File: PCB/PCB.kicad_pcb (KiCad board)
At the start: 2 copper layers, 85 x 55 mm, 32 parts, among them IC2 AP33771CFBZ-13-FA01, IC3 LT8609EMSE#PBF, IC4 AP63203WU-7, J3 UJ20-C-V-SMT-TR-68, Q1 PSMN2R6-30YLC,115, Q2 PSMN2R6-30YLC,115

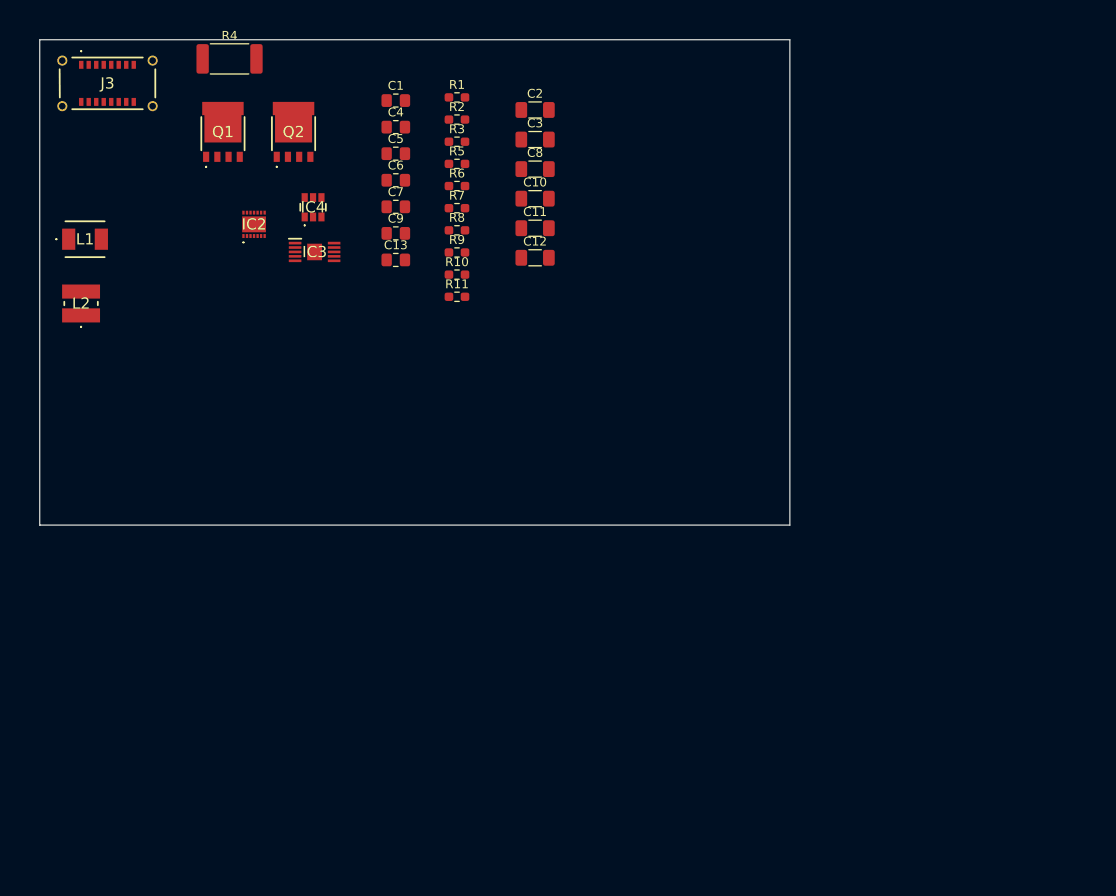
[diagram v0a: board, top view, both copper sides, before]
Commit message: backup power rail pcb
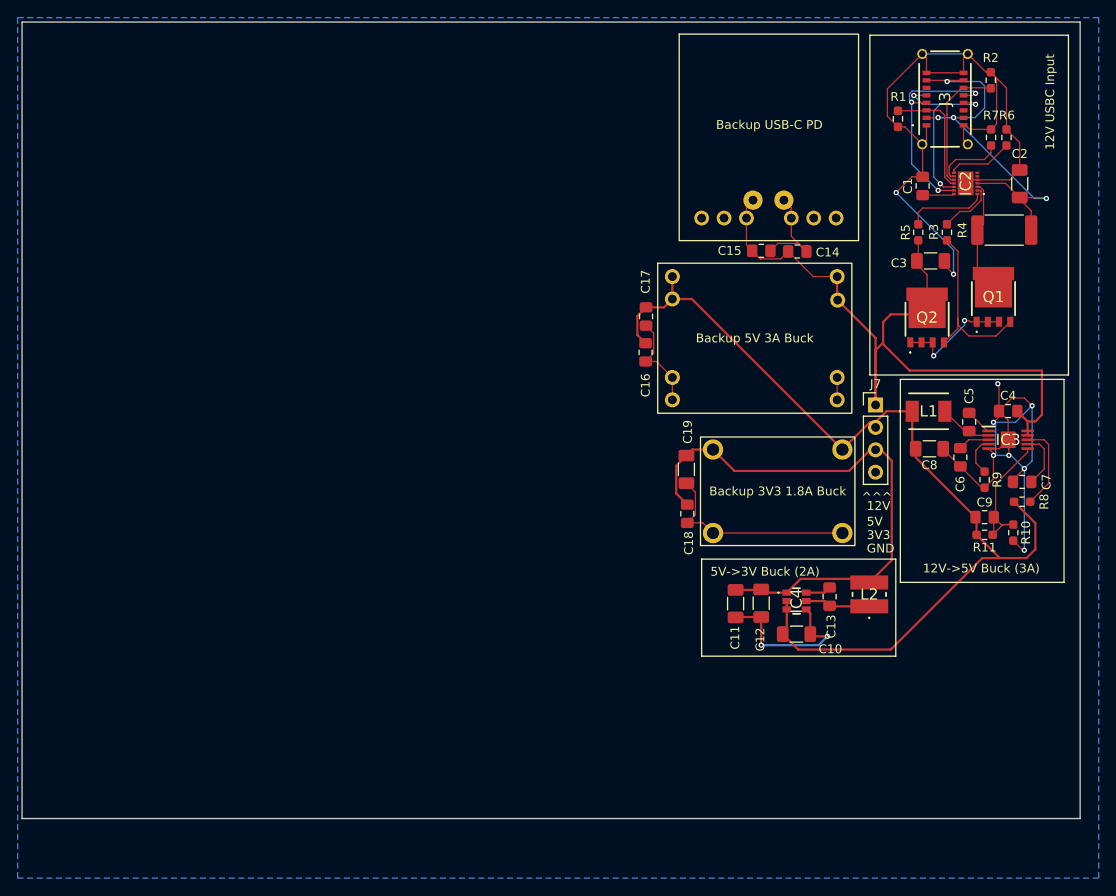
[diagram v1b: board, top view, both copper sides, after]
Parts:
- added C14: 0.1uF, Capacitor_SMD:C_0805_2012Metric_Pad1.18x1.45mm_HandSolder, F.Cu at (100.8, 39.0)
- added C15: 47uF, Capacitor_SMD:C_0805_2012Metric_Pad1.18x1.45mm_HandSolder, F.Cu at (96.8, 38.9)
- added C16: 0.1uF, Capacitor_SMD:C_0805_2012Metric_Pad1.18x1.45mm_HandSolder, F.Cu at (83.7, 50.4)
- added C17: 47uF, Capacitor_SMD:C_0805_2012Metric_Pad1.18x1.45mm_HandSolder, F.Cu at (83.7, 46.4)
- added C18: 0.1uF, Capacitor_SMD:C_0805_2012Metric_Pad1.18x1.45mm_HandSolder, F.Cu at (88.4, 68.7)
- added C19: 22uF, Capacitor_SMD:C_1206_3216Metric_Pad1.33x1.80mm_HandSolder, F.Cu at (88.3, 63.7)
- added J6: USBC_Power_Breakout, SpinnyKitty:USBC_POWER_BREAKOUT, F.Cu at (97.6, 33.2)
- added J7: ~, Connector_PinHeader_2.54mm:PinHeader_1x04_P2.54mm_Vertical, F.Cu at (109.7, 56.4)
- added U3: ~, SpinnyKitty:5V 3A Buck, F.Cu at (96.0, 48.8)
- added U4: ~, SpinnyKitty:3V3 1.8A Buck, F.Cu at (98.6, 66.2)
- C13: value 100nF -> 0.1uF
- moved L1 97.6 mm to (115.7, 57.1)
- moved L2 95.2 mm to (109.0, 77.9)
- moved J3 94.9 mm to (117.6, 21.7), turned to 90 degrees
- moved R4 89.9 mm to (124.3, 36.6), turned to 180 degrees
- moved Q1 89.3 mm to (123.1, 44.3)
- moved IC3 81.4 mm to (124.7, 60.3)
- moved IC2 80.8 mm to (119.9, 31.3), turned to 90 degrees
- moved C7 77.5 mm to (126.3, 65.1)
- moved C4 76.5 mm to (124.7, 57.1), turned to 180 degrees
- moved Q2 74.8 mm to (115.6, 46.6)
- moved C9 74.1 mm to (122.1, 69.1)
- moved C5 71.7 mm to (120.3, 58.3), turned to -90 degrees
- moved C6 71.3 mm to (119.3, 62.3), turned to 90 degrees
- moved R8 71.0 mm to (126.3, 67.4)
- moved IC4 70.7 mm to (100.8, 78.6), turned to -90 degrees
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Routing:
- net GND: track 0.00 -> 217.6 mm, vias 0 -> 11
- net +5V: track 0.00 -> 112.1 mm
- net +12V: track 0.00 -> 84.3 mm
- net +3V3: track 0.00 -> 64.1 mm
- net /VBUS: track 0.00 -> 48.8 mm, vias 0 -> 4
- net /DP: track 0.00 -> 25.0 mm, vias 0 -> 3
- net /DN: track 0.00 -> 21.6 mm, vias 0 -> 3
- net /GATE_DRV: track 0.00 -> 20.6 mm
- net Net-(IC3-FB): track 0.00 -> 16.8 mm
- net /IC_CC2: track 0.00 -> 15.0 mm
- net /IC_CC1: track 0.00 -> 13.9 mm
- net /VBUS_SW_IN: track 0.00 -> 13.6 mm
- net /FET_MID: track 0.00 -> 13.5 mm, vias 0 -> 2
- net /POWER GOOD: track 0.00 -> 9.95 mm
- net Net-(IC2-VOUT): track 0.00 -> 9.28 mm
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- added copper zone on B.Cu, net GND
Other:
- board size 85 x 55 mm -> 119.9 x 90.3 mm
- board text added: "12V"
- board text added: "12V USBC Input"
- board text added: "12V->5V Buck (3A)"
- board text added: "3V3"
- board text added: "5V"
- board text added: "5V->3V Buck (2A)"
- board text added: "GND"
- board text added: "^^^"
